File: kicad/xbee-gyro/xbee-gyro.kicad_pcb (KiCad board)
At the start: 2 copper layers, 69.2 x 61.6 mm, 18 parts, among them J1 IMU_in, J2 IMU, J3 XBee, SW1 Reset, U1 XBEE-S2C, U2 XC6216D_SOT89

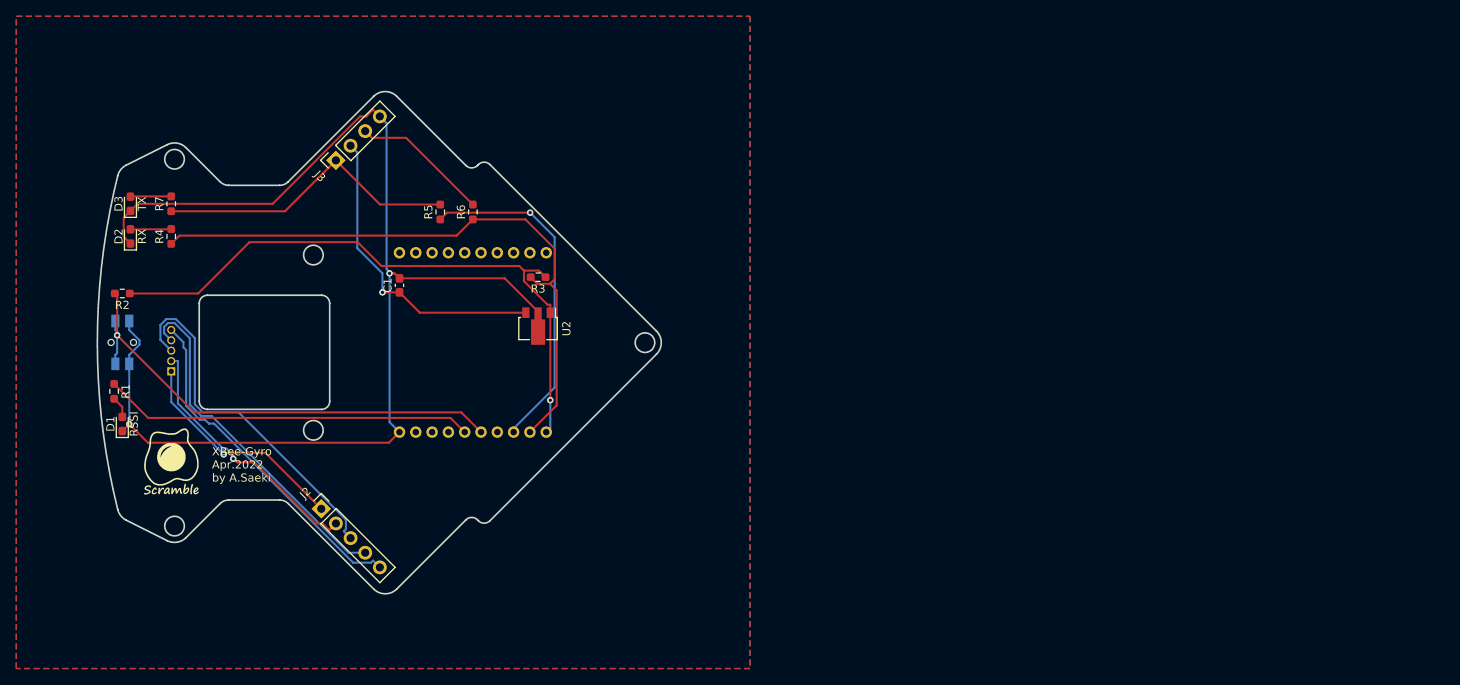
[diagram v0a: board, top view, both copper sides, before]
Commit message: no message
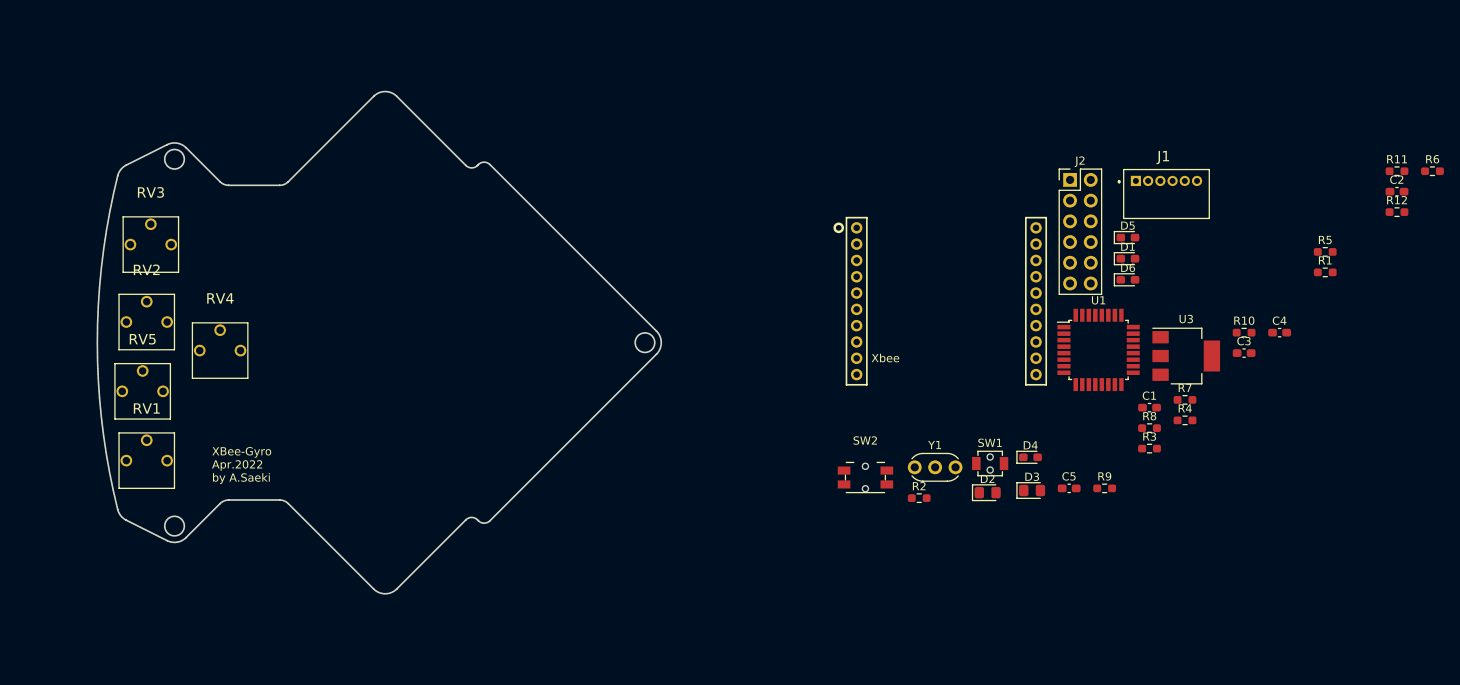
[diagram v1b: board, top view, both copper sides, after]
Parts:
- removed G***: LOGO, LOGO
- removed J3: XBee, Connector_PinSocket_2.54mm:PinSocket_1x04_P2.54mm_Vertical
- added C2: 0.1u, Capacitor_SMD:C_0603_1608Metric_Pad1.08x0.95mm_HandSolder, F.Cu at (204.3, 96.5)
- added C3: 10u, Capacitor_SMD:C_0603_1608Metric_Pad1.08x0.95mm_HandSolder, F.Cu at (185.6, 116.3)
- added C4: 10u, Capacitor_SMD:C_0603_1608Metric_Pad1.08x0.95mm_HandSolder, F.Cu at (189.9, 113.8)
- added C5: 10u, Capacitor_SMD:C_0603_1608Metric_Pad1.08x0.95mm_HandSolder, F.Cu at (164.1, 132.9)
- added D4: RSSI, LED_SMD:LED_0603_1608Metric_Pad1.05x0.95mm_HandSolder, F.Cu at (159.4, 129.1)
- added D5: RX, LED_SMD:LED_0603_1608Metric_Pad1.05x0.95mm_HandSolder, F.Cu at (171.3, 102.1)
- added D6: TX, LED_SMD:LED_0603_1608Metric_Pad1.05x0.95mm_HandSolder, F.Cu at (171.3, 107.3)
- added R10: 10k, Resistor_SMD:R_0603_1608Metric_Pad0.98x0.95mm_HandSolder, F.Cu at (185.6, 113.8)
- added R11: 10k, Resistor_SMD:R_0603_1608Metric_Pad0.98x0.95mm_HandSolder, F.Cu at (204.3, 94.0)
- added R12: 470, Resistor_SMD:R_0603_1608Metric_Pad0.98x0.95mm_HandSolder, F.Cu at (204.3, 99.0)
- added R8: 10k, Resistor_SMD:R_0603_1608Metric_Pad0.98x0.95mm_HandSolder, F.Cu at (174.0, 125.5)
- added R9: 470, Resistor_SMD:R_0603_1608Metric_Pad0.98x0.95mm_HandSolder, F.Cu at (168.5, 132.9)
- added RV1: 20K, 0.main.robot:Trim-GF063P, F.Cu at (51.0, 129.5)
- added RV2: 20K, 0.main.robot:Trim-GF063P, F.Cu at (51.0, 112.5)
- added RV3: 20K, 0.main.robot:Trim-GF063P, F.Cu at (51.5, 103.0)
- added RV4: 20K, 0.main.robot:Trim-GF063P, F.Cu at (60.0, 116.0)
- added RV5: 20K, 0.main.robot:Trim-GF063P, F.Cu at (50.5, 121.0)
- added SW2: Reset, 0.main.robot:THAU13-AB-R, F.Cu at (139.2, 131.6)
- added U3: AZ1117CH-3.3, Package_TO_SOT_SMD:SOT-223-3_TabPin2, F.Cu at (178.5, 116.7)
- added Y1: 8Mhz, Crystal:Resonator-3Pin_W6.0mm_H3.0mm, F.Cu at (145.2, 130.3)
- C1: value 0.1u -> 10u
- D1: value RSSI -> LED(OSWT1608); footprint LED_SMD:LED_0603_1608Metric_Pad1.05x0.95mm_HandSolder -> 0.main.robot:LED_SMLE13WBC8W1
- D2: value RX -> RSX101VAM-30; footprint LED_SMD:LED_0603_1608Metric_Pad1.05x0.95mm_HandSolder -> Diode_SMD:D_0805_2012Metric_Pad1.15x1.40mm_HandSolder
- D3: value TX -> RSX101VAM-30; footprint LED_SMD:LED_0603_1608Metric_Pad1.05x0.95mm_HandSolder -> Diode_SMD:D_0805_2012Metric_Pad1.15x1.40mm_HandSolder
- J1: value IMU_in -> Trimmer; footprint Connector_PinHeader_1.27mm:PinHeader_1x05_P1.27mm_Vertical -> 0.main.robot:JSTS6B-ZRLFSN; moved to F.Cu
- J2: value IMU -> Conn_01x12; footprint Connector_PinSocket_2.54mm:PinSocket_1x05_P2.54mm_Vertical -> Connector_PinHeader_2.54mm:PinHeader_2x06_P2.54mm_Vertical
- R1: value 470 -> 47k
- R2, R3: value 10k -> 47k
- R6: value 10k -> 470
- R7: value 470 -> 10k
- SW1: value Reset -> RESET; footprint 0.main.robot:THAU13-AB-R -> 0.main.robot:TVAF06-A020B-R; moved to F.Cu
- U1: value XBEE-S2C -> ATmega328P-AU; footprint 0.main.robot:XBEE-S2C -> Package_QFP:TQFP-32_7x7mm_P0.8mm; moved to F.Cu
- U2: value XC6216D_SOT89 -> XBEE-S2C; footprint Package_TO_SOT_SMD:SOT-89-3 -> 0.main.robot:XBEE-S2C
- moved R1 149.3 mm to (195.6, 106.4), turned to 0 degrees
- moved R7 126.7 mm to (178.3, 122.0), turned to 0 degrees
- moved R4 126.4 mm to (178.3, 124.6), turned to 0 degrees
- moved D1 125.0 mm to (171.3, 104.7), turned to 0 degrees
- moved J1 120.6 mm to (172.3, 95.2)
- moved R6 117.8 mm to (208.7, 94.0), turned to 0 degrees
- moved D3 116.1 mm to (159.6, 133.2), turned to 0 degrees
- moved D2 109.7 mm to (154.1, 133.4), turned to 0 degrees
- moved R5 108.7 mm to (195.6, 103.9), turned to 0 degrees
- moved SW1 107.5 mm to (154.4, 129.9), turned to 0 degrees
- moved R2 100.9 mm to (145.8, 134.1), turned to 0 degrees
- moved J2 100.3 mm to (164.2, 95.1), turned to 0 degrees
- moved C1 93.2 mm to (174.0, 123.0), turned to 0 degrees
- moved U1 87.8 mm to (167.8, 115.9), turned to 0 degrees
- moved R3 77.9 mm to (174.0, 128.0), turned to 0 degrees
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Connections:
- C1 pad 1: +5V -> Vcc1
- D2 pad 1: GND -> Vcc1
- D2 pad 2: Net-(D2-Pad2) -> ICSP_5
- D3 pad 1: GND -> Vcc1
- J1 pad 5: Net-(J1-Pad5) -> Line5
- J2 pad 1: Net-(J1-Pad1) -> Vcc1
- J2 pad 2: Net-(J1-Pad2) -> +5V
- J2 pad 3: Net-(J1-Pad3) -> unconnected-(J2-Pad3)
- J2 pad 4: Net-(J1-Pad4) -> GND
- J2 pad 5: Net-(J1-Pad5) -> XBee_1
- R1 pad 2: Net-(D1-Pad2) -> Vcc1
- R2 pad 1: Net-(R2-Pad1) -> Vcc1
- R2 pad 2: Net-(R2-Pad2) -> OLED_SCL
- R3 pad 1: Net-(R2-Pad1) -> Vcc1
- R3 pad 2: Net-(R3-Pad2) -> OLED_SDA
- R4 pad 1: Net-(R3-Pad2) -> Net-(R4-Pad1)
- R4 pad 2: Net-(D2-Pad2) -> Net-(D1-Pad2)
- R5 pad 1: Net-(R5-Pad1) -> ICSP_5
- R5 pad 2: Net-(J3-Pad1) -> Vcc1
- R6 pad 1: Net-(R3-Pad2) -> Net-(R6-Pad1)
- R7 pad 1: Net-(J3-Pad1) -> Net-(C4-Pad1)
- R7 pad 2: Net-(D3-Pad2) -> Net-(R7-Pad2)
- SW1 pad 1: Net-(R2-Pad2) -> GND
- SW1 pad 2: GND -> ICSP_5
- U1 pad 1: Net-(R2-Pad1) -> unconnected-(U1-Pad1)
- U1 pad 10: GND -> Net-(R4-Pad1)
- U1 pad 15: unconnected-(U1-Pad15) -> ICSP_4
- U1 pad 16: unconnected-(U1-Pad16) -> ICSP_1
- U1 pad 17: unconnected-(U1-Pad17) -> ICSP_3
- U1 pad 18: unconnected-(U1-Pad18) -> Vcc1
- U1 pad 19: unconnected-(U1-Pad19) -> Line5
- U1 pad 2: Net-(R3-Pad2) -> unconnected-(U1-Pad2)
- U1 pad 3: Net-(R5-Pad1) -> GND
- U1 pad 4: unconnected-(U1-Pad4) -> Vcc1
- U1 pad 5: Net-(R2-Pad2) -> GND
- U1 pad 6: Net-(R1-Pad1) -> Vcc1
- U1 pad 7: unconnected-(U1-Pad7) -> Net-(U1-Pad7)
- U1 pad 8: unconnected-(U1-Pad8) -> Net-(U1-Pad8)
- U2 pad 1: Net-(R2-Pad1) -> Net-(C4-Pad1)
- U2 pad 2: GND -> Net-(R11-Pad1)
- U2 pad 3: +5V -> Net-(R10-Pad1)
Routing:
- net GND: track 150.4 -> 0.00 mm, vias 2 -> 0
- net Net-(R2-Pad1): track 76.9 -> 0.00 mm, vias 1 -> 0
- net Net-(R3-Pad2): track 76.9 -> 0.00 mm
- net Net-(R2-Pad2): track 60.2 -> 0.00 mm, vias 1 -> 0
- net Net-(R1-Pad1): track 45.4 -> 0.00 mm
- net Net-(J1-Pad3): track 44.4 -> 0.00 mm
- net Net-(J1-Pad4): track 43.3 -> 0.00 mm
- net Net-(J1-Pad5): track 42.3 -> 0.00 mm
- net Net-(R5-Pad1): track 41.6 -> 0.00 mm, vias 1 -> 0
- net +5V: track 38.2 -> 0.00 mm, vias 1 -> 0
- net Net-(J3-Pad1): track 37.8 -> 0.00 mm
- net Net-(J1-Pad2): track 32.4 -> 0.00 mm, vias 1 -> 0
- net Net-(J1-Pad1): track 27.7 -> 0.00 mm, vias 1 -> 0
- net Net-(D4-Pad2): track 16.9 -> 0.00 mm
- net Net-(D3-Pad2): track 5.02 -> 0.00 mm
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- removed copper zone on B.Cu, net GND
- removed copper zone on F.Cu, net GND
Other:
- outline, holes or cut-outs redrawn

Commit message: add: xbee-gyro
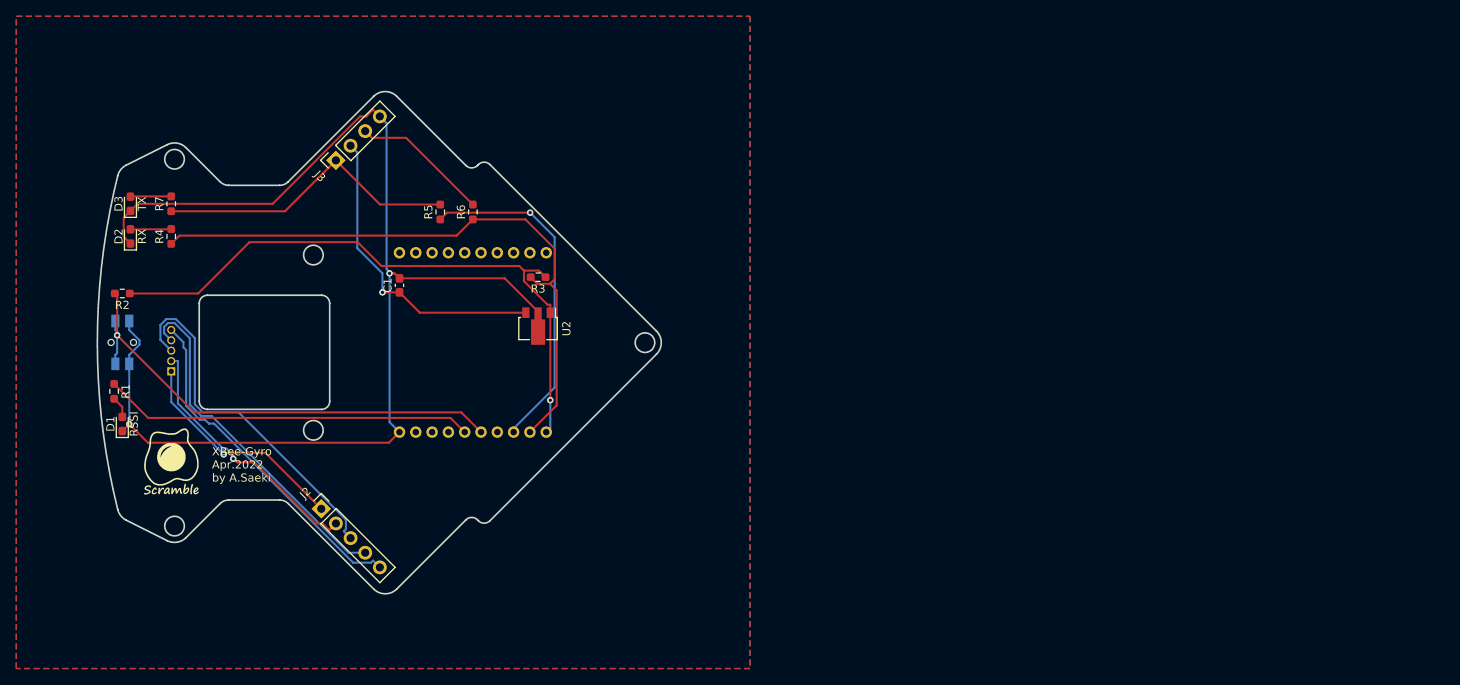
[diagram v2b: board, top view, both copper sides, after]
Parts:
- removed C2: 0.1u, Capacitor_SMD:C_0603_1608Metric_Pad1.08x0.95mm_HandSolder
- removed C3, C4, C5: 10u, Capacitor_SMD:C_0603_1608Metric_Pad1.08x0.95mm_HandSolder
- removed D4: RSSI, LED_SMD:LED_0603_1608Metric_Pad1.05x0.95mm_HandSolder
- removed D5: RX, LED_SMD:LED_0603_1608Metric_Pad1.05x0.95mm_HandSolder
- removed D6: TX, LED_SMD:LED_0603_1608Metric_Pad1.05x0.95mm_HandSolder
- removed R10, R11, R8: 10k, Resistor_SMD:R_0603_1608Metric_Pad0.98x0.95mm_HandSolder
- removed R12, R9: 470, Resistor_SMD:R_0603_1608Metric_Pad0.98x0.95mm_HandSolder
- removed RV1, RV2, RV3, RV4, RV5: 20K, 0.main.robot:Trim-GF063P
- removed SW2: Reset, 0.main.robot:THAU13-AB-R
- removed U3: AZ1117CH-3.3, Package_TO_SOT_SMD:SOT-223-3_TabPin2
- removed Y1: 8Mhz, Crystal:Resonator-3Pin_W6.0mm_H3.0mm
- added G***: LOGO, LOGO, F.Cu at (54.0, 130.0)
- added J3: XBee, Connector_PinSocket_2.54mm:PinSocket_1x04_P2.54mm_Vertical, F.Cu at (74.2, 92.7)
- C1: value 10u -> 0.1u
- D1: value LED(OSWT1608) -> RSSI; footprint 0.main.robot:LED_SMLE13WBC8W1 -> LED_SMD:LED_0603_1608Metric_Pad1.05x0.95mm_HandSolder
- D2: value RSX101VAM-30 -> RX; footprint Diode_SMD:D_0805_2012Metric_Pad1.15x1.40mm_HandSolder -> LED_SMD:LED_0603_1608Metric_Pad1.05x0.95mm_HandSolder
- D3: value RSX101VAM-30 -> TX; footprint Diode_SMD:D_0805_2012Metric_Pad1.15x1.40mm_HandSolder -> LED_SMD:LED_0603_1608Metric_Pad1.05x0.95mm_HandSolder
- J1: value Trimmer -> IMU_in; footprint 0.main.robot:JSTS6B-ZRLFSN -> Connector_PinHeader_1.27mm:PinHeader_1x05_P1.27mm_Vertical; moved to B.Cu
- J2: value Conn_01x12 -> IMU; footprint Connector_PinHeader_2.54mm:PinHeader_2x06_P2.54mm_Vertical -> Connector_PinSocket_2.54mm:PinSocket_1x05_P2.54mm_Vertical
- R1: value 47k -> 470
- R2, R3: value 47k -> 10k
- R6: value 470 -> 10k
- R7: value 10k -> 470
- SW1: value RESET -> Reset; footprint 0.main.robot:TVAF06-A020B-R -> 0.main.robot:THAU13-AB-R; moved to B.Cu
- U1: value ATmega328P-AU -> XBEE-S2C; footprint Package_QFP:TQFP-32_7x7mm_P0.8mm -> 0.main.robot:XBEE-S2C; moved to B.Cu
- U2: value XBEE-S2C -> XC6216D_SOT89; footprint 0.main.robot:XBEE-S2C -> Package_TO_SOT_SMD:SOT-89-3
- moved R1 149.3 mm to (47.0, 121.0), turned to -90 degrees
- moved R7 126.7 mm to (54.0, 98.0), turned to 90 degrees
- moved R4 126.4 mm to (54.0, 102.0), turned to 90 degrees
- moved D1 125.0 mm to (48.0, 125.0), turned to 90 degrees
- moved J1 120.6 mm to (54.0, 118.5)
- moved R6 117.8 mm to (91.0, 99.0), turned to 90 degrees
- moved D3 116.1 mm to (49.0, 98.0), turned to 90 degrees
- moved D2 109.7 mm to (49.0, 102.0), turned to 90 degrees
- moved R5 108.7 mm to (87.0, 99.0), turned to 90 degrees
- moved SW1 107.5 mm to (48.0, 115.0), turned to -90 degrees
- moved R2 100.9 mm to (48.0, 109.0), turned to 180 degrees
- moved J2 100.3 mm to (72.4, 135.4), turned to 45 degrees
- moved C1 93.2 mm to (82.0, 108.0), turned to 90 degrees
- moved U1 87.8 mm to (80.0, 115.0), turned to 90 degrees
- moved R3 77.9 mm to (99.0, 107.0), turned to 180 degrees
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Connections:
- C1 pad 1: Vcc1 -> +5V
- D2 pad 1: Vcc1 -> GND
- D2 pad 2: ICSP_5 -> Net-(D2-Pad2)
- D3 pad 1: Vcc1 -> GND
- J1 pad 5: Line5 -> Net-(J1-Pad5)
- J2 pad 1: Vcc1 -> Net-(J1-Pad1)
- J2 pad 2: +5V -> Net-(J1-Pad2)
- J2 pad 3: unconnected-(J2-Pad3) -> Net-(J1-Pad3)
- J2 pad 4: GND -> Net-(J1-Pad4)
- J2 pad 5: XBee_1 -> Net-(J1-Pad5)
- R1 pad 2: Vcc1 -> Net-(D1-Pad2)
- R2 pad 1: Vcc1 -> Net-(R2-Pad1)
- R2 pad 2: OLED_SCL -> Net-(R2-Pad2)
- R3 pad 1: Vcc1 -> Net-(R2-Pad1)
- R3 pad 2: OLED_SDA -> Net-(R3-Pad2)
- R4 pad 1: Net-(R4-Pad1) -> Net-(R3-Pad2)
- R4 pad 2: Net-(D1-Pad2) -> Net-(D2-Pad2)
- R5 pad 1: ICSP_5 -> Net-(R5-Pad1)
- R5 pad 2: Vcc1 -> Net-(J3-Pad1)
- R6 pad 1: Net-(R6-Pad1) -> Net-(R3-Pad2)
- R7 pad 1: Net-(C4-Pad1) -> Net-(J3-Pad1)
- R7 pad 2: Net-(R7-Pad2) -> Net-(D3-Pad2)
- SW1 pad 1: GND -> Net-(R2-Pad2)
- SW1 pad 2: ICSP_5 -> GND
- U1 pad 1: unconnected-(U1-Pad1) -> Net-(R2-Pad1)
- U1 pad 10: Net-(R4-Pad1) -> GND
- U1 pad 15: ICSP_4 -> unconnected-(U1-Pad15)
- U1 pad 16: ICSP_1 -> unconnected-(U1-Pad16)
- U1 pad 17: ICSP_3 -> unconnected-(U1-Pad17)
- U1 pad 18: Vcc1 -> unconnected-(U1-Pad18)
- U1 pad 19: Line5 -> unconnected-(U1-Pad19)
- U1 pad 2: unconnected-(U1-Pad2) -> Net-(R3-Pad2)
- U1 pad 3: GND -> Net-(R5-Pad1)
- U1 pad 4: Vcc1 -> unconnected-(U1-Pad4)
- U1 pad 5: GND -> Net-(R2-Pad2)
- U1 pad 6: Vcc1 -> Net-(R1-Pad1)
- U1 pad 7: Net-(U1-Pad7) -> unconnected-(U1-Pad7)
- U1 pad 8: Net-(U1-Pad8) -> unconnected-(U1-Pad8)
- U2 pad 1: Net-(C4-Pad1) -> Net-(R2-Pad1)
- U2 pad 2: Net-(R11-Pad1) -> GND
- U2 pad 3: Net-(R10-Pad1) -> +5V
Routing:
- net GND: track 0.00 -> 150.4 mm, vias 0 -> 2
- net Net-(R2-Pad1): track 0.00 -> 76.9 mm, vias 0 -> 1
- net Net-(R3-Pad2): track 0.00 -> 76.9 mm
- net Net-(R2-Pad2): track 0.00 -> 60.2 mm, vias 0 -> 1
- net Net-(R1-Pad1): track 0.00 -> 45.4 mm
- net Net-(J1-Pad3): track 0.00 -> 44.4 mm
- net Net-(J1-Pad4): track 0.00 -> 43.3 mm
- net Net-(J1-Pad5): track 0.00 -> 42.3 mm
- net Net-(R5-Pad1): track 0.00 -> 41.6 mm, vias 0 -> 1
- net +5V: track 0.00 -> 38.2 mm, vias 0 -> 1
- net Net-(J3-Pad1): track 0.00 -> 37.8 mm
- net Net-(J1-Pad2): track 0.00 -> 32.4 mm, vias 0 -> 1
- net Net-(J1-Pad1): track 0.00 -> 27.7 mm, vias 0 -> 1
- net Net-(J3-Pad3): track 0.00 -> 16.9 mm
- net Net-(D3-Pad2): track 0.00 -> 5.02 mm
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- added copper zone on B.Cu, net GND
- added copper zone on F.Cu, net GND
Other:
- outline, holes or cut-outs redrawn
